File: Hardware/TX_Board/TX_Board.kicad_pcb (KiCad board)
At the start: 4 copper layers, 148 x 98.8 mm, 224 parts, among them IC1 GP2Y1+, IC10 QPA9122TR7, IC11 MAPS-010164-TR0500, IC12 QPA9122TR7, IC13 MAPS-010164-TR0500, IC14 QPA9122TR7, IC2 GP2Y1+, IC3 GP2Y1+, IC4 LT3041ADE#PBF, IC5 LT3099ADE#PBF, IC6 ADPL40502AUJZ-1.5-R7, IC7 MAPS-010164-TR0500, IC8 QPA9122TR7, IC9 MAPS-010164-TR0500, J1 Conn_Coaxial, J10 MM8030-2610RJ3, J11 MM8030-2610RJ3, J12 MM8030-2610RJ3, J13 MM8030-2610RJ3, J14 MM8030-2610RJ3, J15 Conn_Coaxial, J16 MM8030-2610RJ3, J17 MM8030-2610RJ3, J18 Conn_Coaxial, J19 MM8030-2610RJ3, J2 Conn_01x01_Pin, J20 MM8030-2610RJ3, J21 Conn_Coaxial, J22 MM8030-2610RJ3, J23 MM8030-2610RJ3, J24 Conn_Coaxial, J3 Conn_01x01_Pin, J4 Conn_01x01_Pin, J5 Conn_01x01_Pin, J6 Conn_02x12_Odd_Even, J7 Conn_01x03_Socket, J8 Conn_02x08_Odd_Even, J9 MM8030-2610RJ3, U1 SN74HCT138NSR

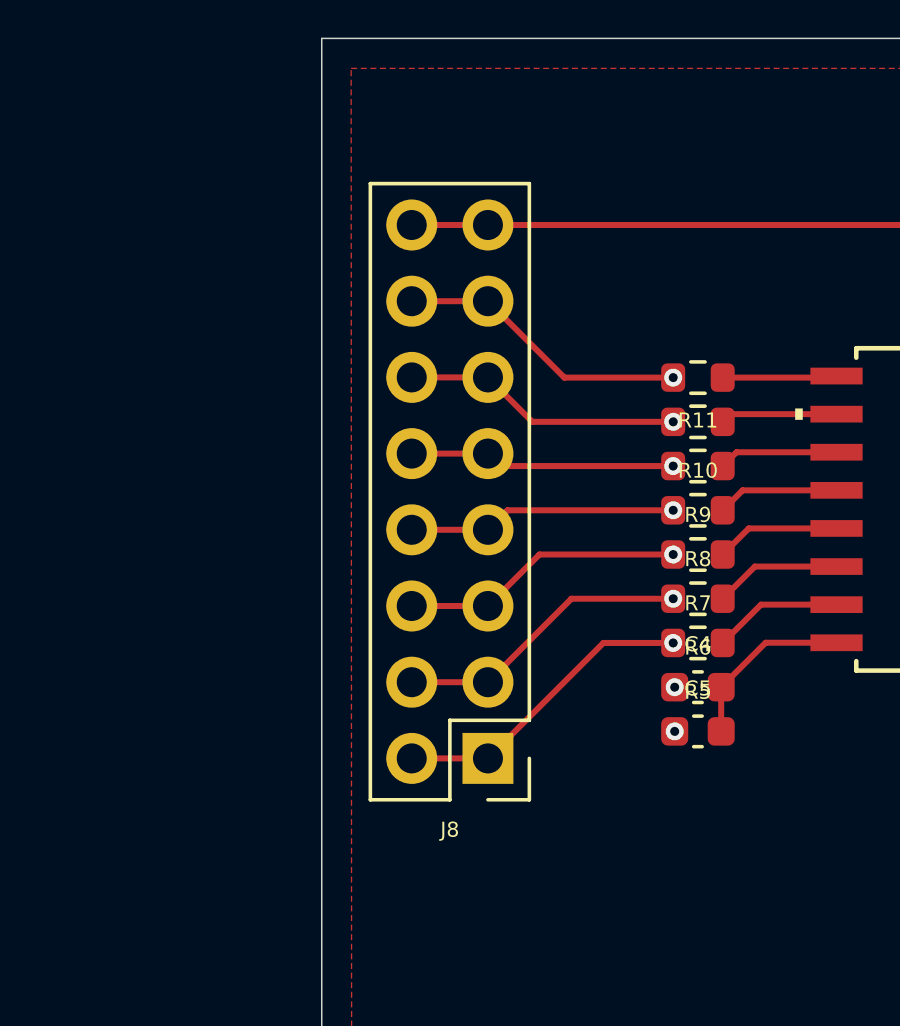
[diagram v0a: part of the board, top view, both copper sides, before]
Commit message: more routing
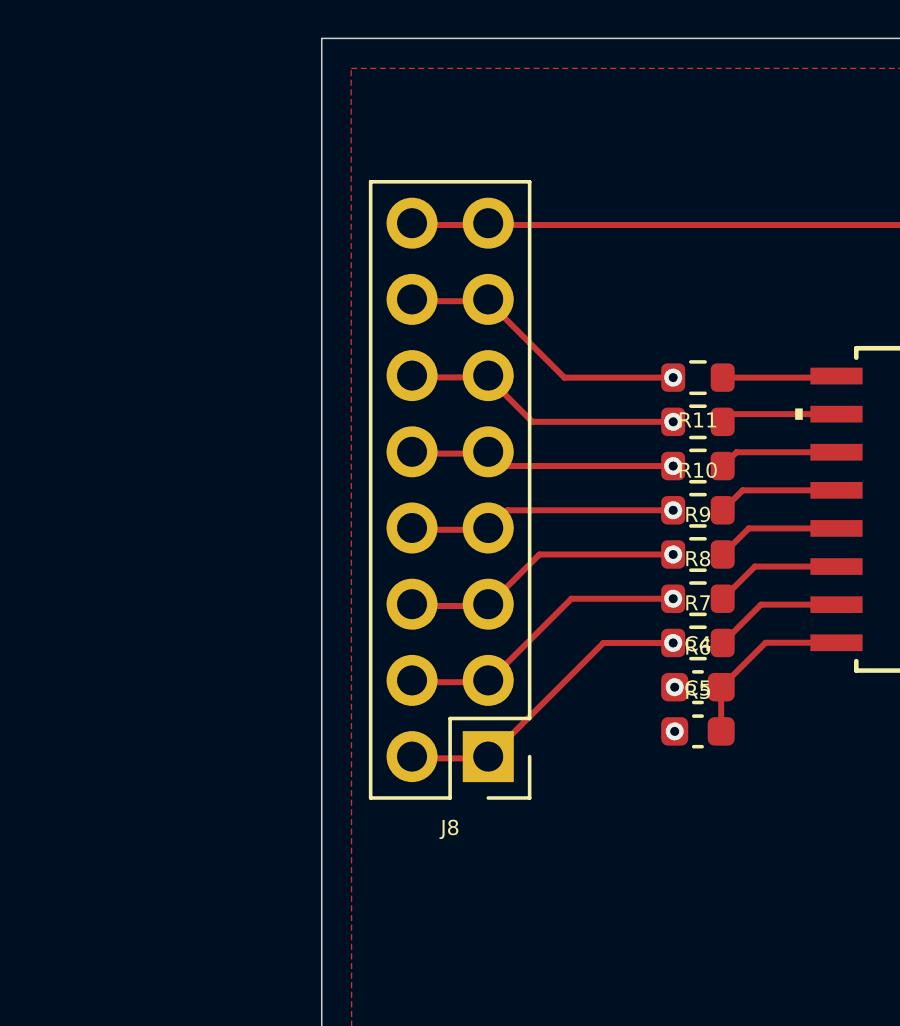
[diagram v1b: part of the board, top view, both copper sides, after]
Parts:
- moved J8 0.06 mm to (87.5, 53.9)
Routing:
- net ATTN_CLK: track 2.54 -> 75.0 mm
- net ATTN_SI: track 2.54 -> 74.6 mm
- net PS_SER_OUT: track 2.54 -> 65.1 mm
- net PS_CLK: track 2.54 -> 61.9 mm
- net PS_SER_IN: track 2.54 -> 61.0 mm
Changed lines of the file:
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@@
 	(footprint "Connector_PinHeader_2.54mm:PinHeader_2x08_P2.54mm_Vertical"
 		(layer "F.Cu")
-		(at 87.5 54 180)
+		(at 87.51 53.94 180)
 		(descr "Through hole straight pin header, 2x08, 2.54mm pitch, double rows")
 		(tags "Through hole pin header THT 2x08 2.54mm double row")
 		(property "Reference" "J8"
-			(at 1.27 -2.38 180)
+			(at 1.27 -2.38 0)
 			(layer "F.SilkS")
 			(effects
@@
 		)
 		(property "Value" "Conn_02x08_Odd_Even"
-			(at 1.27 20.16 180)
+			(at 1.27 20.16 0)
 			(layer "F.Fab")
 			(effects
@@
 		)
 		(property "Datasheet" "~"
-			(at 0 0 180)
+			(at 0 0 0)
 			(layer "F.Fab")
 			(hide yes)
@@
 		)
 		(property "Description" "Generic connector, double row, 02x08, odd/even pin numbering scheme (row 1 odd numbers, row 2 even numbers), script generated (kicad-library-utils/schlib/autogen/connector/)"
-			(at 0 0 180)
+			(at 0 0 0)
 			(layer "F.Fab")
 			(hide yes)
@@
 		)
 		(fp_text user "${REFERENCE}"
-			(at 1.27 8.89 270)
+			(at 1.27 8.89 90)
 			(layer "F.Fab")
 			(effects
@@
 		(fill no)
 		(layer "In1.Cu")
+		(net 48)
 	)
 	(gr_rect
@@
 	)
 	(segment
+		(start 167.12 35.18)
+		(end 174.24 35.18)
+		(width 0.2)
+		(layer "In2.Cu")
+		(net 64)
+	)
+	(segment
+		(start 174.24 35.18)
+		(end 174.4 35.34)
+		(width 0.2)
+		(layer "In2.Cu")
+		(net 64)
+	)
+	(segment
+		(start 125.281 40.371)
+		(end 161.929 40.371)
+		(width 0.2)
+		(layer "In2.Cu")
+		(net 64)
+	)
+	(segment
+		(start 174.4 35.34)
+		(end 174.4 35.975)
+		(width 0.2)
+		(layer "In2.Cu")
+		(net 64)
+	)
+	(segment
+		(start 120.66 35.75)
+		(end 125.281 40.371)
+		(width 0.2)
+		(layer "In2.Cu")
+		(net 64)
+	)
+	(segment
+		(start 161.929 40.371)
+		(end 167.12 35.18)
+		(width 0.2)
+		(layer "In2.Cu")
+		(net 64)
+	)
+	(segment
 		(start 123.2 33.21)
 		(end 123.2 35.75)
@@
 	)
 	(segment
+		(start 177.4 35.15)
+		(end 177.4 35.975)
+		(width 0.2)
+		(layer "In2.Cu")
+		(net 65)
+	)
+	(segment
+		(start 123.2 35.75)
+		(end 127.42 39.97)
+		(width 0.2)
+		(layer "In2.Cu")
+		(net 65)
+	)
+	(segment
+		(start 166.83 34.45)
+		(end 176.7 34.45)
+		(width 0.2)
+		(layer "In2.Cu")
+		(net 65)
+	)
+	(segment
+		(start 161.31 39.97)
+		(end 166.83 34.45)
+		(width 0.2)
+		(layer "In2.Cu")
+		(net 65)
+	)
+	(segment
+		(start 127.42 39.97)
+		(end 161.31 39.97)
+		(width 0.2)
+		(layer "In2.Cu")
+		(net 65)
+	)
+	(segment
+		(start 176.7 34.45)
+		(end 177.4 35.15)
+		(width 0.2)
+		(layer "In2.Cu")
+		(net 65)
+	)
+	(segment
 		(start 125.74 33.21)
 		(end 125.74 35.75)
@@
 	)
 	(segment
+		(start 181.85 33.97)
+		(end 166.53 33.97)
+		(width 0.2)
+		(layer "In2.Cu")
+		(net 66)
+	)
+	(segment
+		(start 129.44 39.45)
+		(end 125.74 35.75)
+		(width 0.2)
+		(layer "In2.Cu")
+		(net 66)
+	)
+	(segment
+		(start 183.4 35.975)
+		(end 183.4 35.52)
+		(width 0.2)
+		(layer "In2.Cu")
+		(net 66)
+	)
+	(segment
+		(start 166.53 33.97)
+		(end 161.05 39.45)
+		(width 0.2)
+		(layer "In2.Cu")
+		(net 66)
+	)
+	(segment
+		(start 161.05 39.45)
+		(end 129.44 39.45)
+		(width 0.2)
+		(layer "In2.Cu")
+		(net 66)
+	)
+	(segment
+		(start 183.4 35.52)
+		(end 181.85 33.97)
+		(width 0.2)
+		(layer "In2.Cu")
+		(net 66)
+	)
+	(segment
 		(start 204.48 91.01)
 		(end 197.6 91.01)
@@
 	)
 	(segment
+		(start 130.82 35.75)
+		(end 133.718 38.648)
+		(width 0.2)
+		(layer "In2.Cu")
+		(net 68)
+	)
+	(segment
+		(start 166.01 33.168)
+		(end 194.893 33.168)
+		(width 0.2)
+		(layer "In2.Cu")
+		(net 68)
+	)
+	(segment
+		(start 160.53 38.648)
+		(end 166.01 33.168)
+		(width 0.2)
+		(layer "In2.Cu")
+		(net 68)
+	)
+	(segment
+		(start 194.893 33.168)
+		(end 198.4 36.675)
+		(width 0.2)
+		(layer "In2.Cu")
+		(net 68)
+	)
+	(segment
+		(start 133.718 38.648)
+		(end 160.53 38.648)
+		(width 0.2)
+		(layer "In2.Cu")
+		(net 68)
+	)
+	(segment
 		(start 213.22 92.08)
 		(end 213.3 92)
@@
 	)
 	(segment
+		(start 192.294 33.569)
+		(end 195.4 36.675)
+		(width 0.2)
+		(layer "In2.Cu")
+		(net 70)
+	)
+	(segment
+		(start 131.579 39.049)
+		(end 160.8839 39.049)
+		(width 0.2)
+		(layer "In2.Cu")
+		(net 70)
+	)
+	(segment
+		(start 160.8839 39.049)
+		(end 166.3639 33.569)
+		(width 0.2)
+		(layer "In2.Cu")
+		(net 70)
+	)
+	(segment
+		(start 128.28 35.75)
+		(end 131.579 39.049)
+		(width 0.2)
+		(layer "In2.Cu")
+		(net 70)
+	)
+	(segment
+		(start 166.3639 33.569)
+		(end 192.294 33.569)
+		(width 0.2)
+		(layer "In2.Cu")
+		(net 70)
+	)
+	(segment
 		(start 215.32 88.095)
 		(end 214.85 87.625)
@@
 		(priority 5)
 		(connect_pads
-			(clearance 0.2)
+			(clearance 0.5)
 		)
 		(min_thickness 0.25)
